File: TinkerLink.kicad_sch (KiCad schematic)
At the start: 28 parts, among them J1 Conn_01x06_Pin, Q1 IRF4905S, Q2 MMBT2222A, Q3 SQS411ENW-T1_GE3, SW1 TS-061D-250D4-P, U1 ESP-01F-2M, U2 ME6211C33M5, U3 AP63203WU

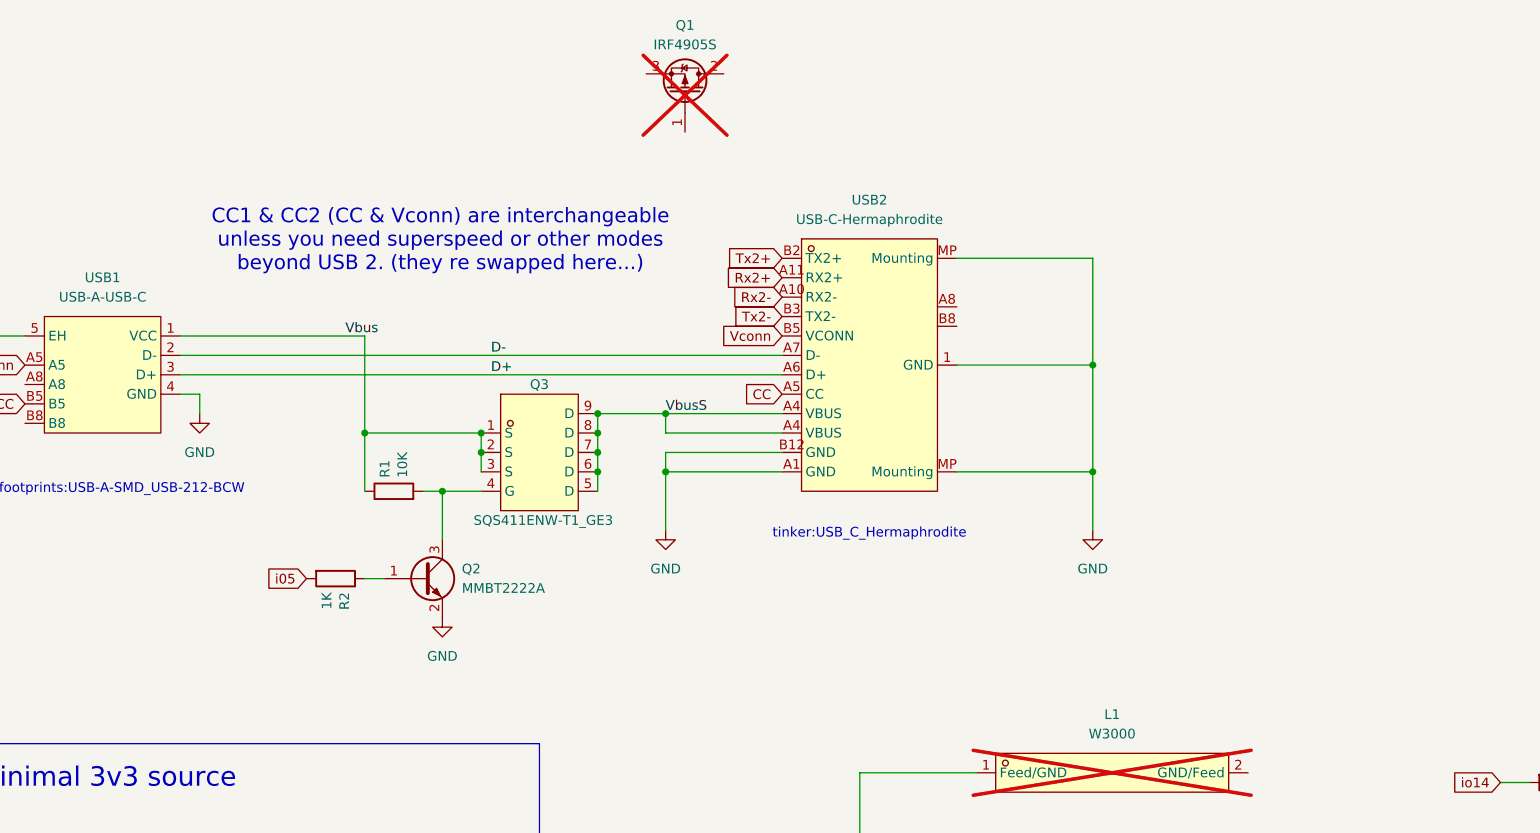
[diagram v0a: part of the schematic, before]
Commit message: Dual FETs
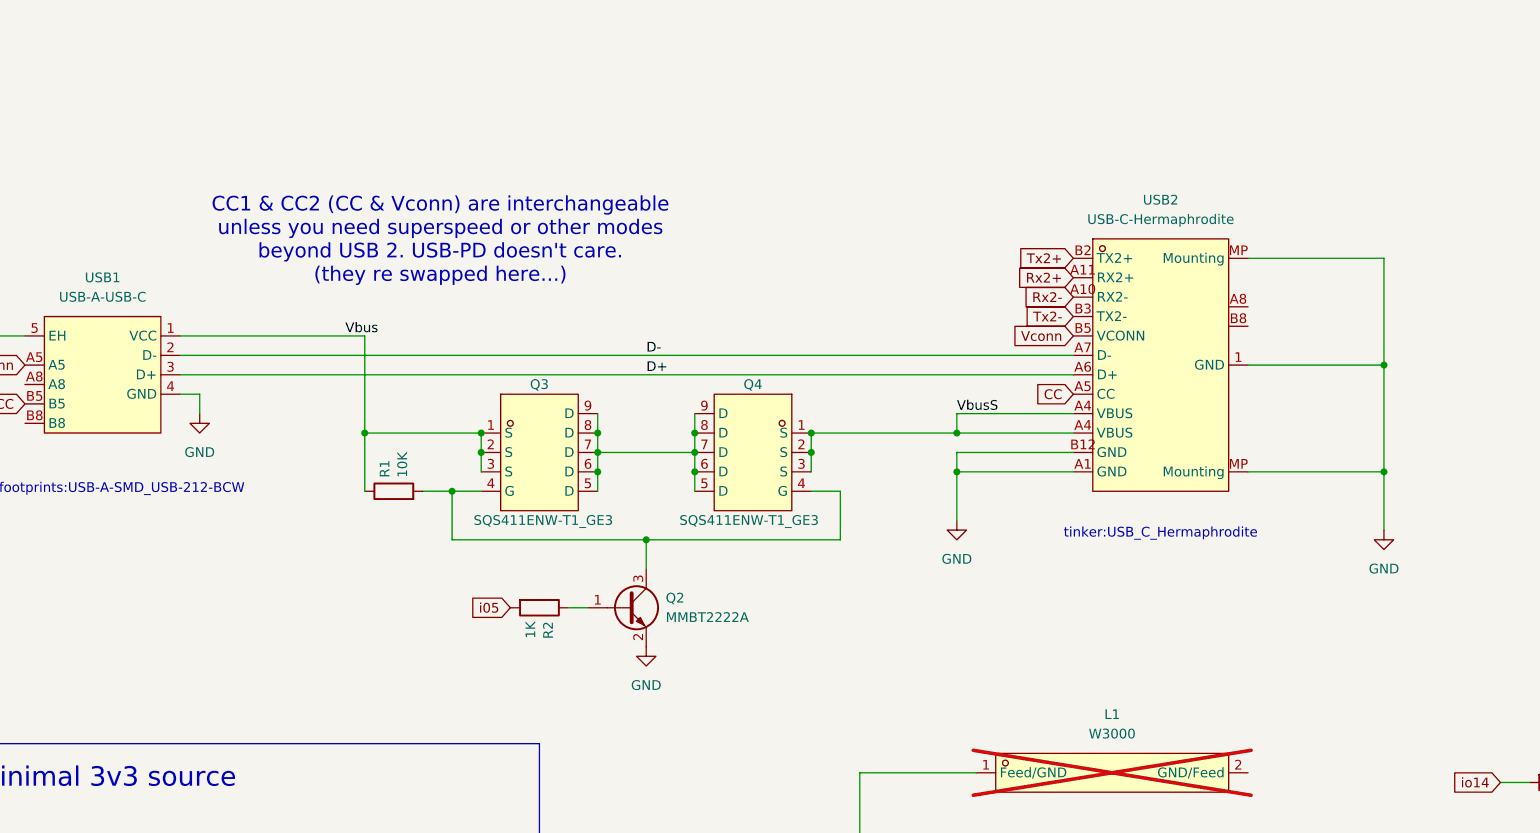
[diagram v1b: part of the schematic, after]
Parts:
- removed Q1: IRF4905S, Package_TO_SOT_SMD:TO-252-2, symbol Transistor_FET:IRF4905
- added Q4: SQS411ENW-T1_GE3, LCSCfootprints:POWERPAK-1212-8_L3.1-W3.1-P0.65-LS3.3-BL, symbol C3279469:SQS411ENW-T1_GE3
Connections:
- net VbusS: now also Q4.1 (S), Q4.2 (S), Q4.3 (S); no longer Q3.5 (D), Q3.6 (D), Q3.7 (D), Q3.8 (D), Q3.9 (D)
- net at Q2.3 (C), Q3.4 (G), R1.2: now also Q4.4 (G)
- new net: Q3.5 (D), Q3.6 (D), Q3.7 (D), Q3.8 (D), Q3.9 (D), Q4.5 (D), Q4.6 (D), Q4.7 (D), Q4.8 (D), Q4.9 (D)
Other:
- note added: "CC1 & CC2 (CC & Vconn) are interchangeable unless you need superspeed or other modes beyond USB 2. USB-PD doesn't care. (they re swapped here...)"
- note removed: "CC1 & CC2 (CC & Vconn) are interchangeable unless you need superspeed or other modes beyond USB 2. (they re swapped here...)"
- moved on the sheet: Q2, R2, USB2
